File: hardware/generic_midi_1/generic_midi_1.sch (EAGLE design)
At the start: 26 parts, among them IC1 MEGA168/328, IC2 RFM12

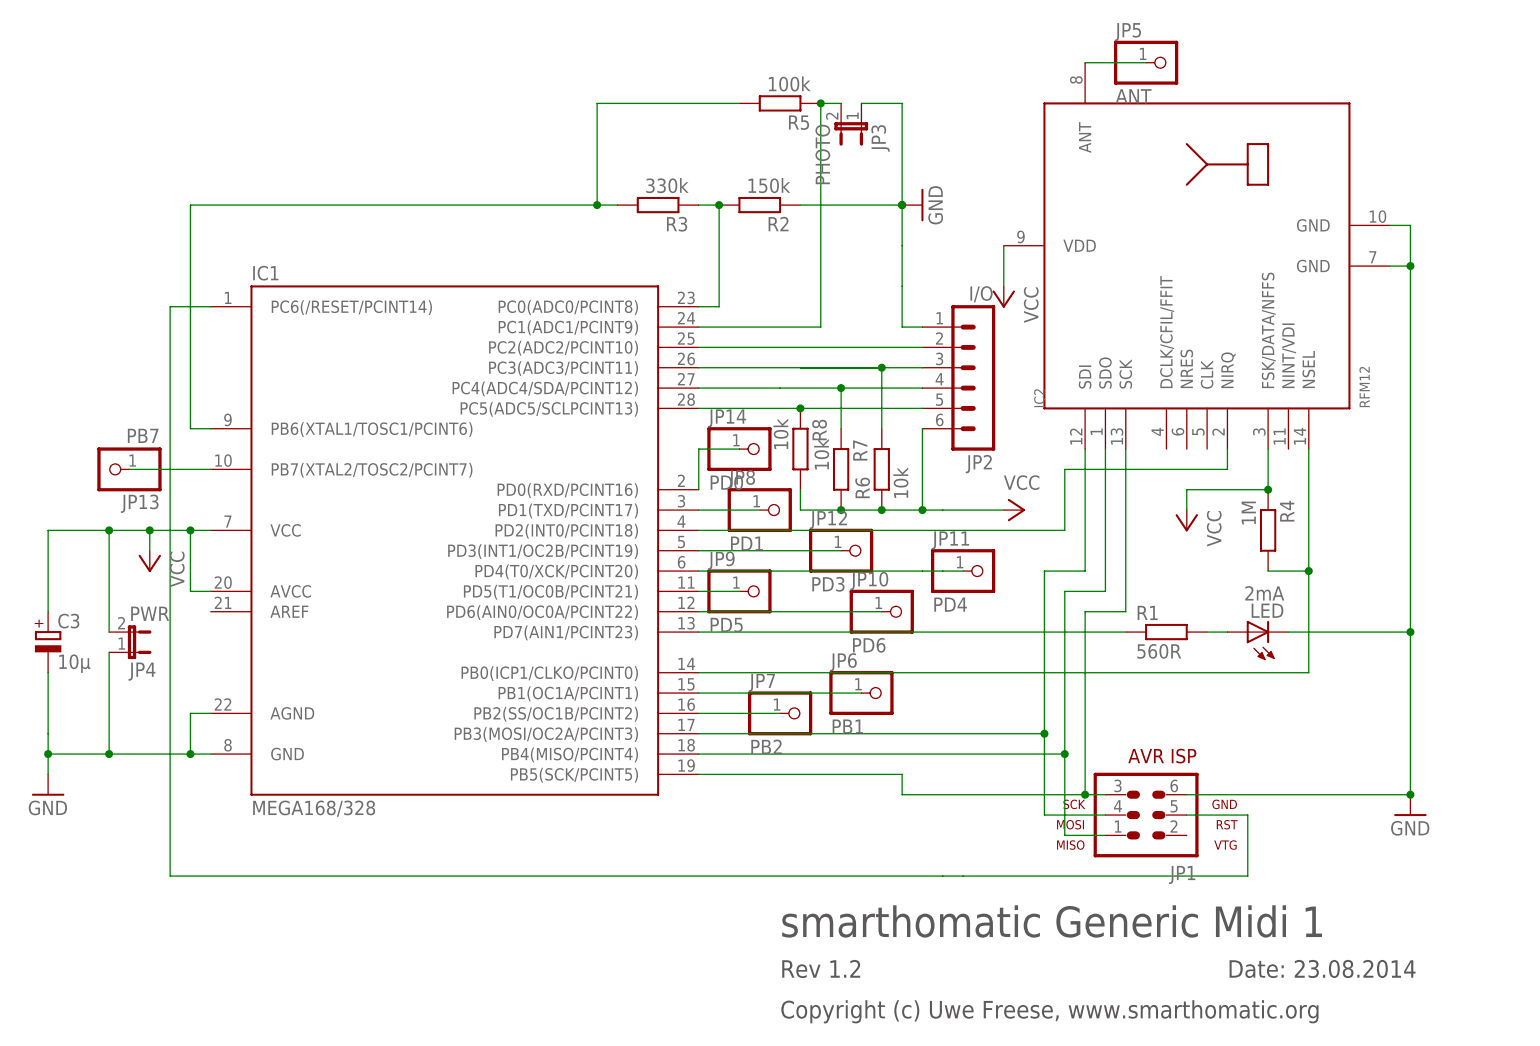
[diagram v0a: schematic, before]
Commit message: test
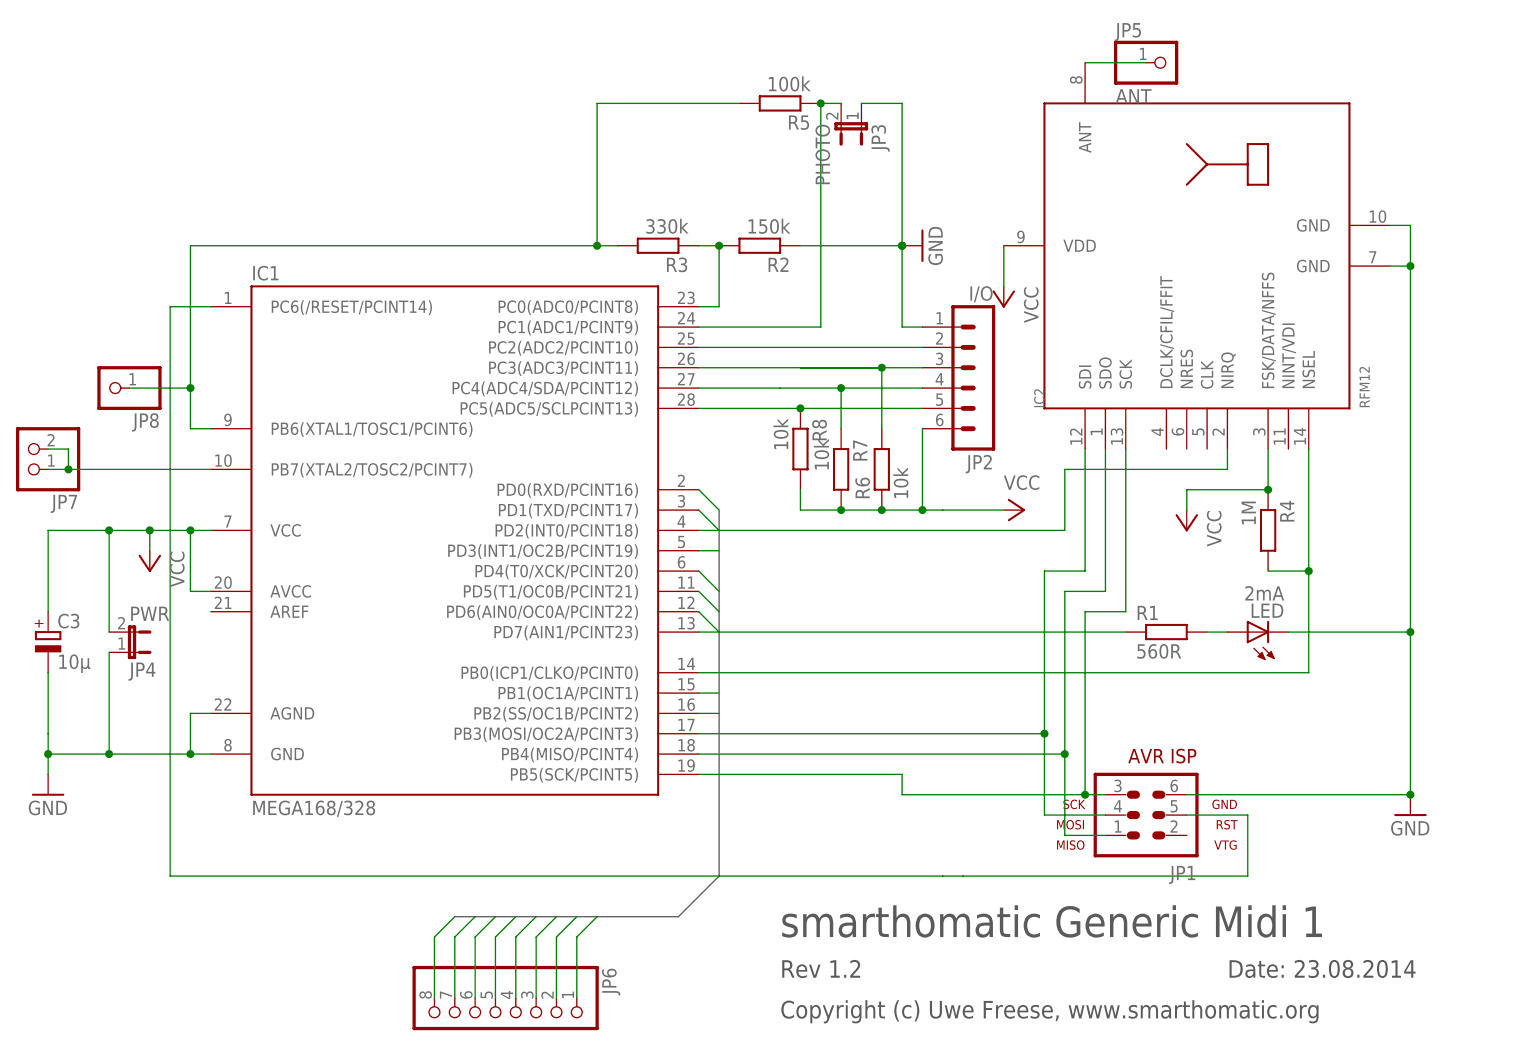
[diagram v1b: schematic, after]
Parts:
- removed JP10: PD6, pinhead:PINHD-1X1
- removed JP11: PD4, pinhead:PINHD-1X1
- removed JP12: PD3, pinhead:PINHD-1X1
- removed JP13: PB7, pinhead:PINHD-1X1
- removed JP14: PD0, pinhead:PINHD-1X1
- removed JP9: PD5, pinhead:PINHD-1X1
- JP6: value PB1 -> (none); device pinhead:PINHD-1X1 -> pinhead:PINHD-1X8
- JP7: value PB2 -> (none); device pinhead:PINHD-1X1 -> pinhead:PINHD-1X2
- JP8: value PD1 -> (none)
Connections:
- removed net N$16: IC1.PD6(AIN0/OC0A/PCINT22), JP10.1
- removed net N$17: IC1.PB1(OC1A/PCINT1), JP6.1
- removed net N$19: IC1.PB2(SS/OC1B/PCINT2), JP7.1
- removed net N$20: IC1.PD1(TXD/PCINT17), JP8.1
- removed net N$22: IC1.PD4(T0/XCK/PCINT20), JP11.1
- removed net N$23: IC1.PD3(INT1/OC2B/PCINT19), JP12.1
- removed net N$25: IC1.PB7(XTAL2/TOSC2/PCINT7), JP13.1
- removed net N$26: IC1.PD0(RXD/PCINT16), JP14.1
- new net IO0: IC1.PD1(TXD/PCINT17), JP6.1
- new net IO1: IC1.PD0(RXD/PCINT16), JP6.2
- new net IO2: IC1.PD3(INT1/OC2B/PCINT19), JP6.3
- new net IO3: IC1.PD4(T0/XCK/PCINT20), JP6.4
- new net IO4: IC1.PD5(T1/OC0B/PCINT21), JP6.5
- new net IO5: IC1.PD6(AIN0/OC0A/PCINT22), JP6.6
- new net IO6: IC1.PB1(OC1A/PCINT1), JP6.7
- new net IO7: IC1.PB2(SS/OC1B/PCINT2), JP6.8
- net N$14: now also IC1.PB7(XTAL2/TOSC2/PCINT7), JP7.1, JP7.2; no longer IC1.PD5(T1/OC0B/PCINT21), JP9.1
- net N$24: now also JP8.1
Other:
- moved on the sheet: JP8, R2, R3
